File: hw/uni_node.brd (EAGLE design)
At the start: 18 x 13.5 mm, 4 parts, among them U1 TINY45, X1 BUS

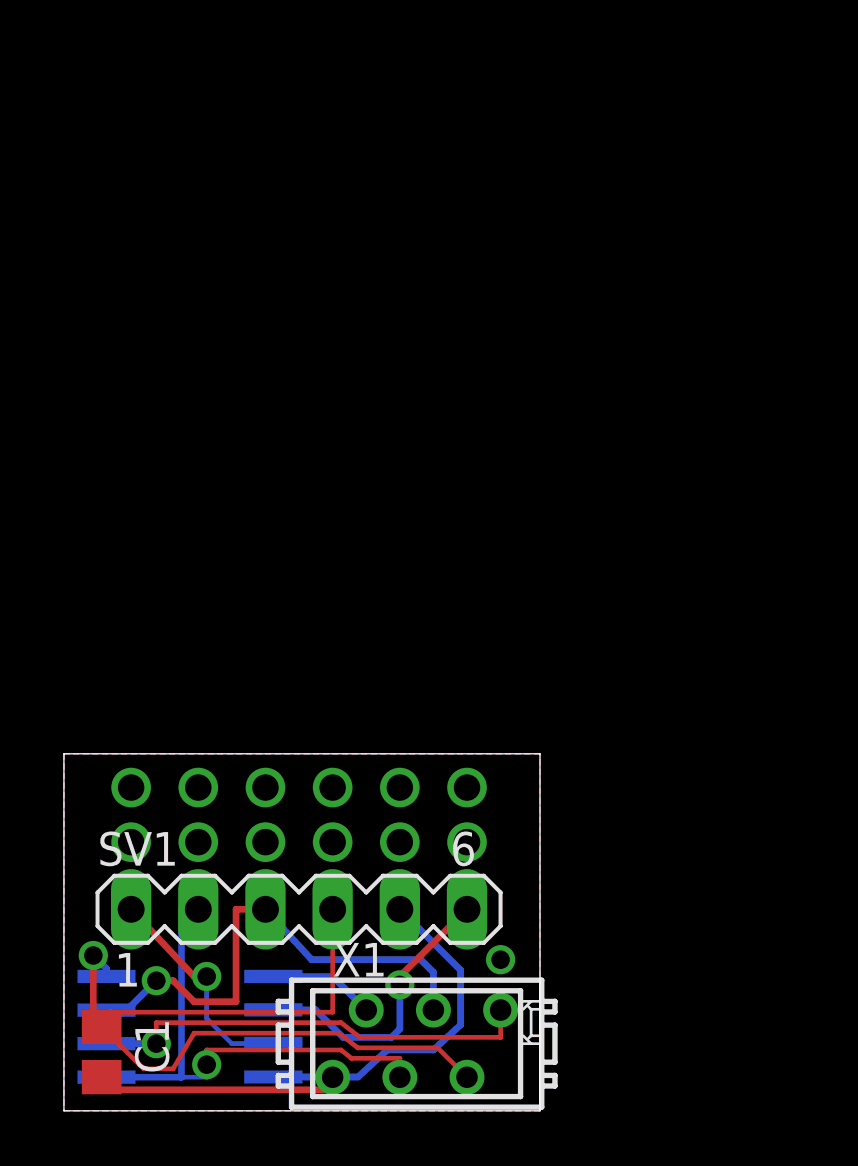
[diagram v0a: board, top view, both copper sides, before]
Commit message: -
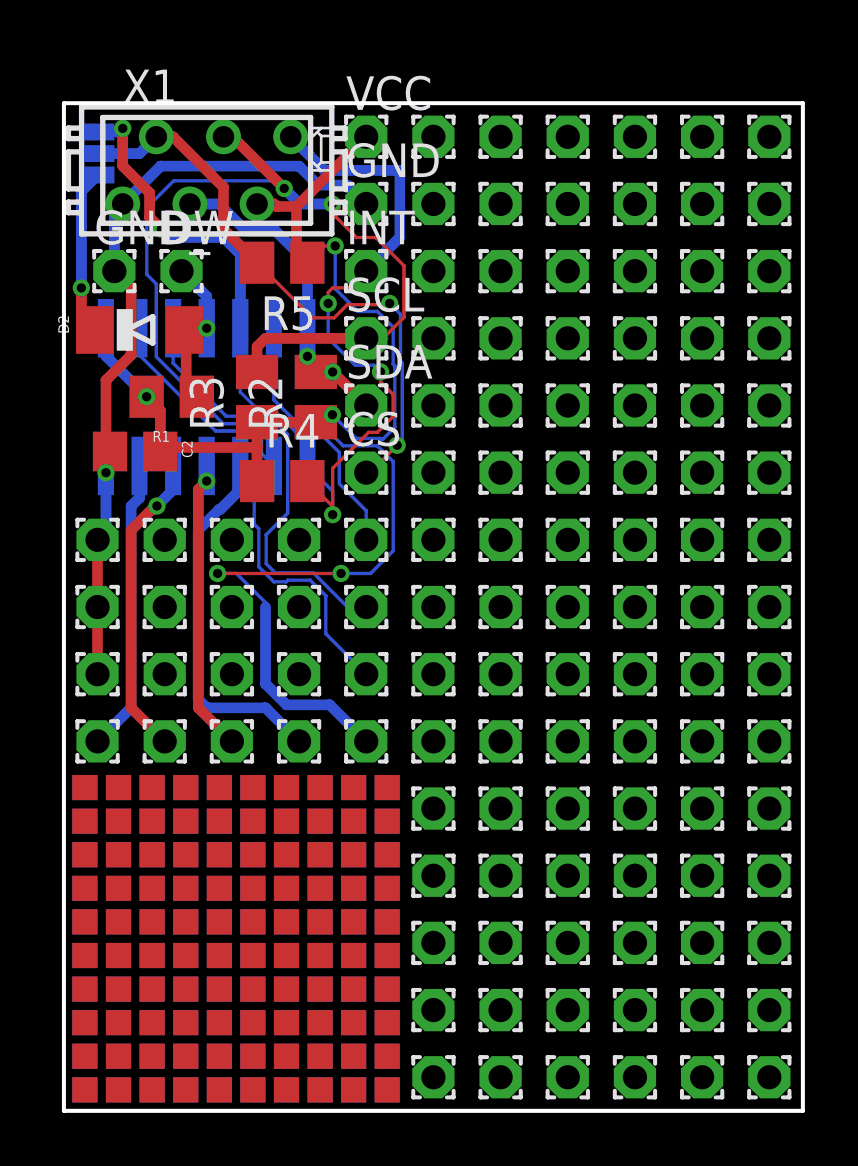
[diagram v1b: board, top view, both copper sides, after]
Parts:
- removed C1: 100n, rcl:C0805
- removed SV1: (no value), con-lstb:MA06-1
- removed U1: TINY45, avr-7:SOIC8
- added C2: 100n, rcl:C0805
- added CS, DW, GND, GND_, INT, INT0, PA0, PA1, PA2, PA3, PA7, PAD1, PAD10, PAD100, PAD101, PAD102, PAD11, PAD12, PAD13, PAD14, PAD15, PAD16, PAD17, PAD18, PAD19, PAD2, PAD20, PAD21, PAD22, PAD23, PAD24, PAD25, PAD26, PAD27, PAD28, PAD29, PAD3, PAD30, PAD31, PAD32, PAD33, PAD34, PAD35, PAD36, PAD37, PAD38, PAD39, PAD4, PAD40, PAD41, PAD42, PAD43, PAD44, PAD45, PAD46, PAD47, PAD48, PAD49, PAD5, PAD50, PAD51, PAD52, PAD53, PAD54, PAD55, PAD56, PAD57, PAD58, PAD59, PAD6, PAD60, PAD61, PAD62, PAD63, PAD64, PAD65, PAD66, PAD67, PAD68, PAD69, PAD7, PAD70, PAD71, PAD72, PAD73, PAD74, PAD75, PAD76, PAD77, PAD78, PAD79, PAD8, PAD80, PAD81, PAD82, PAD83, PAD84, PAD85, PAD86, PAD87, PAD88, PAD89, PAD9, PAD90, PAD91, PAD92, PAD93, PAD94, PAD95, PAD96, PAD97, PAD98, PAD99, PB0, PB1, SCL, SDA, VCC: (no value), wirepad:1,6/0,9
- added D2: (no value), diode:MINIMELF
- added IC1: TINY84 or TINY841, avr-7:SOIC14
- added J_CS: (no value), SparkFun-Jumpers:SMT-JUMPER_3_1-NC_PASTE_NO-SILK
- added R1, R2, R3, R4, R5: 10k, rcl:M0805
- moved X1 34.0 mm to (5.40, 35.6)
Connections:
- removed net INT_MISO: U1.6, X1.1
- removed net PB3: SV1.6, U1.2
- removed net PB4: SV1.1, U1.3
- removed net RESET: U1.1, X1.5
- removed net SCL_SCK: SV1.3, U1.7, X1.3
- removed net SDA_MOSI: SV1.2, U1.5, X1.4
- new net BUS_INT: IC1.8, INT.1, R4.2, X1.1
- new net BUS_P5: CS.1, J_CS.2, R5.2, X1.5
- new net BUS_RESET: D2.C, J_CS.3
- new net BUS_SCL: IC1.9, R3.2, SCL.1, X1.3
- new net BUS_SDA: IC1.7, R2.2, SDA.1, X1.4
- new net DW: D2.A, DW.1, IC1.4, R1.2
- new net INT0: IC1.5, INT0.1, J_CS.1
- new net PA0: IC1.13, PA0.1
- new net PA1: IC1.12, PA1.1
- new net PA2: IC1.11, PA2.1
- new net PA3: IC1.10, PA3.1
- new net PA7: IC1.6, PA7.1
- new net PB0: IC1.2, PB0.1
- new net PB1: IC1.3, PB1.1
- net GND: now also C2.2, GND.1, GND_.1, IC1.14, PAD100.1, PAD101.1, PAD102.1; no longer C1.2, SV1.5, U1.4
- net VCC: now also C2.1, IC1.1, R1.1, R2.1, R3.1, R4.1, R5.1, VCC.1; no longer C1.1, SV1.4, U1.8
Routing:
- net BUS_SCL: track 0.00 -> 36.1 mm, vias 0 -> 2
- net PA7: track 0.00 -> 28.6 mm, vias 0 -> 2
- net BUS_INT: track 0.00 -> 25.6 mm, vias 0 -> 3
- net BUS_P5: track 0.00 -> 22.5 mm, vias 0 -> 2
- net INT0: track 0.00 -> 22.4 mm, vias 0 -> 2
- net SDA_MOSI: track 19.9 -> 0.00 mm, vias 1 -> 0
- net SCL_SCK: track 19.1 -> 0.00 mm, vias 1 -> 0
- net PB0: track 0.00 -> 18.3 mm
- net INT_MISO: track 16.9 -> 0.00 mm, vias 1 -> 0
- net PB1: track 0.00 -> 16.5 mm
- net PA3: track 0.00 -> 14.0 mm
- net BUS_SDA: track 0.00 -> 12.1 mm, vias 0 -> 2
- net PA1: track 0.00 -> 11.6 mm, vias 0 -> 1
- net PA2: track 0.00 -> 11.1 mm, vias 0 -> 1
- net PA0: track 0.00 -> 11.1 mm
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- removed copper zone on layer 1, net GND
- removed copper zone on layer 16, net GND
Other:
- board size 18 x 13.5 mm -> 27.9 x 38.1 mm
